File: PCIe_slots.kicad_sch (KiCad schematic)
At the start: 33 parts, among them J1 PCIe_x16_CPU

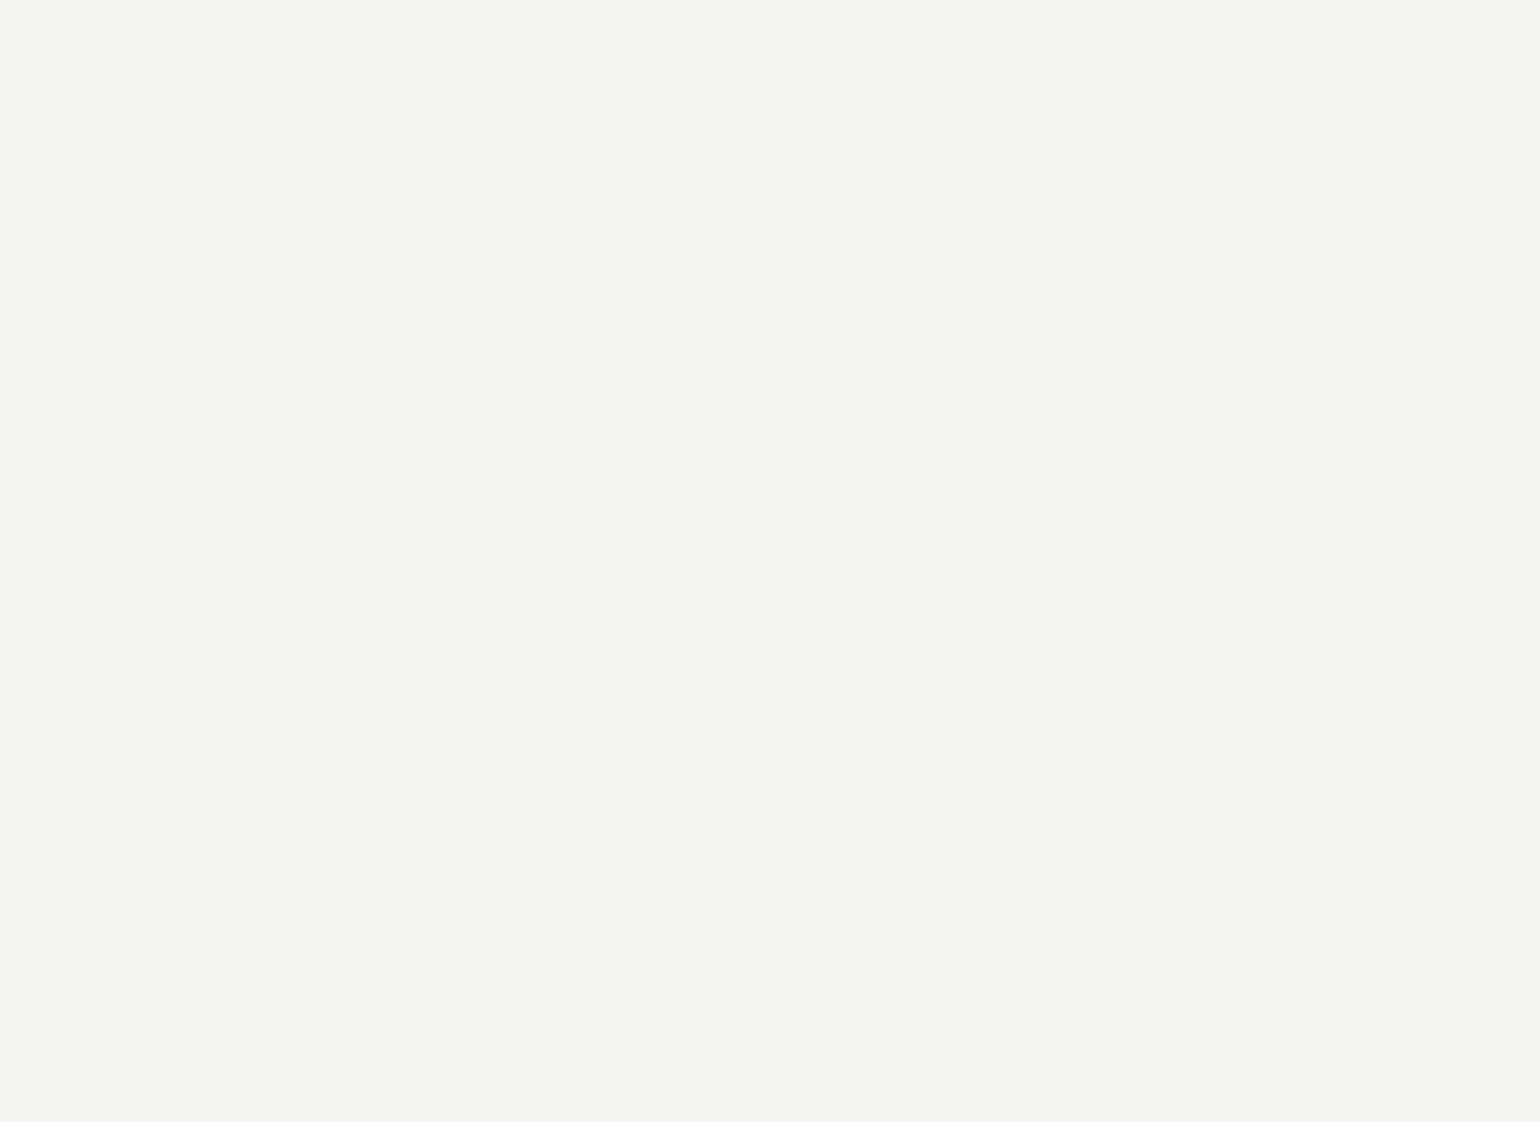
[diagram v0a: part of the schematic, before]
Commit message: idek what i changed anymore but there's a bunch of new stuff lol
iirc i did some more misc cpu pins and a bunch of pch pcie stuff
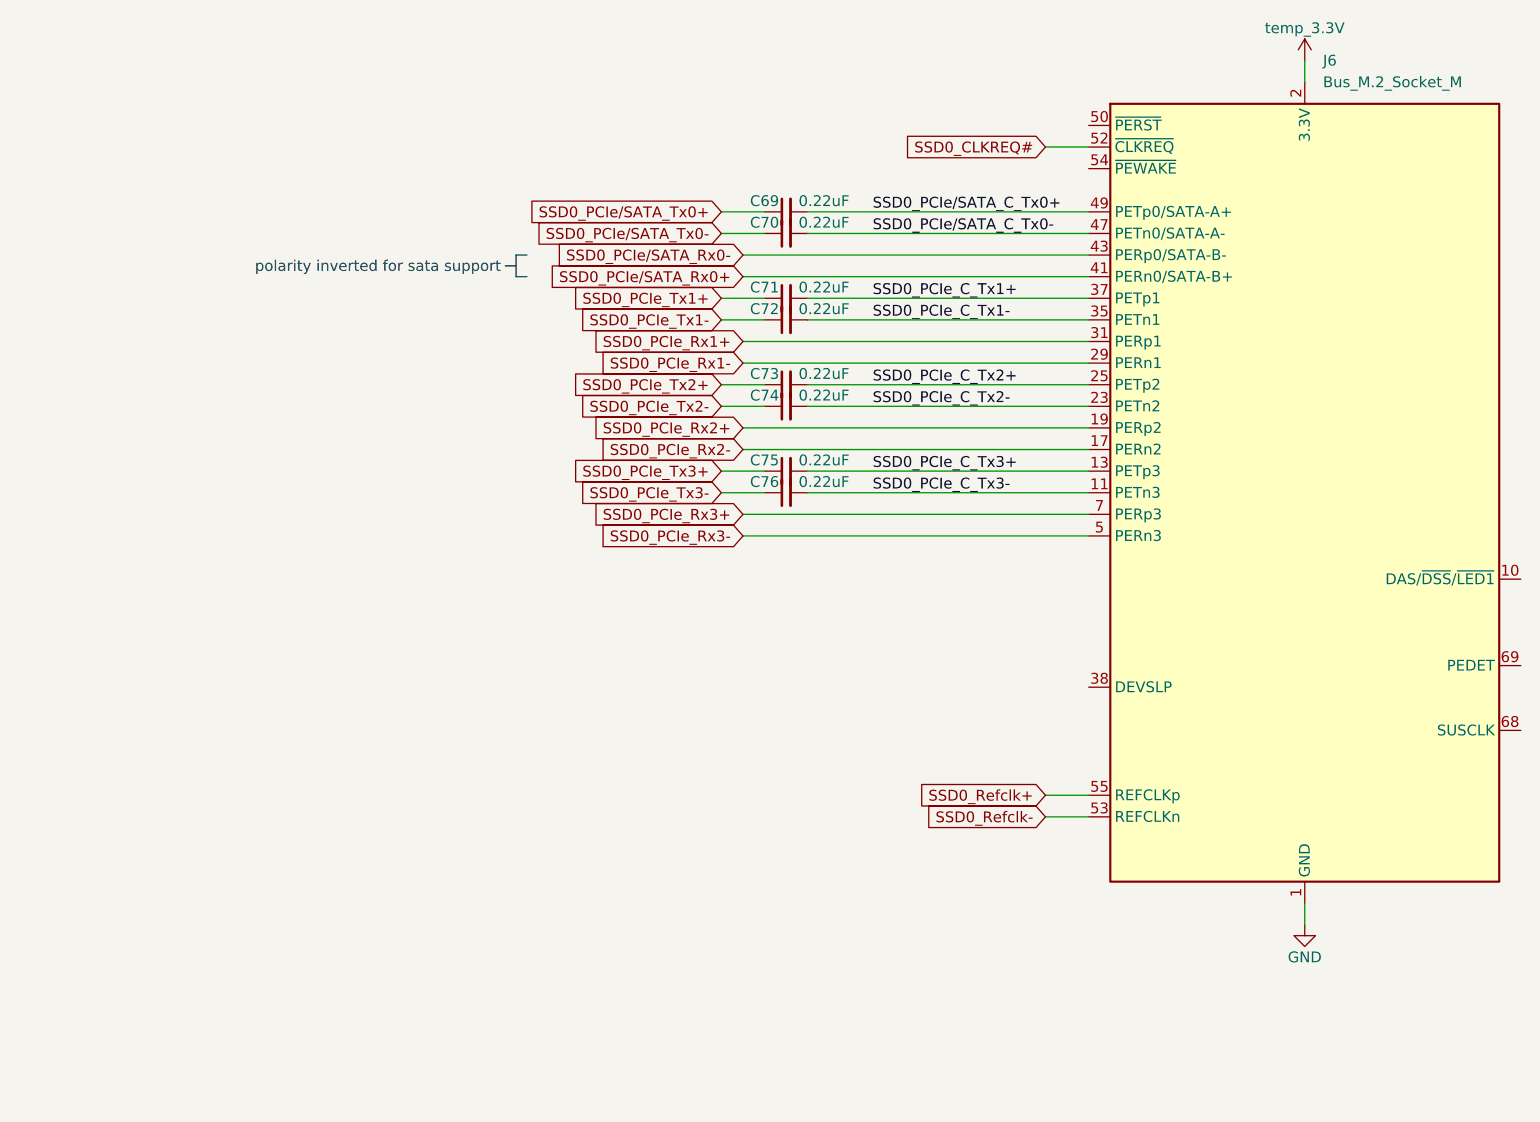
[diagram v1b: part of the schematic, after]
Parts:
- added C69, C70, C71, C72, C73, C74, C75, C76: 0.22uF, Capacitor_SMD:C_0402_1005Metric, symbol Device:C_Small
- added J6: Bus_M.2_Socket_M, A-my-stuff:m-key, symbol Connector:Bus_M.2_Socket_M
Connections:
- net GND: now also J6.1 (GND), J6.15 (GND), J6.21 (GND), J6.27 (GND), J6.3 (GND), J6.33 (GND), J6.39 (GND), J6.45 (GND), J6.51 (GND), J6.57 (GND), J6.71 (GND), J6.73 (GND), J6.75 (GND), J6.9 (GND)
- net temp_3.3V: now also J6.12 (3.3V), J6.14 (3.3V), J6.16 (3.3V), J6.18 (3.3V), J6.2 (3.3V), J6.4 (3.3V), J6.70 (3.3V), J6.72 (3.3V), J6.74 (3.3V)
- new net SSD0_CLKREQ#: J6.52 (~{CLKREQ})
- new net SSD0_PCIe/SATA_C_Tx0+: C69.2, J6.49 (PETp0/SATA-A+)
- new net SSD0_PCIe/SATA_C_Tx0-: C70.2, J6.47 (PETn0/SATA-A-)
- new net SSD0_PCIe/SATA_Rx0+: J6.41 (PERn0/SATA-B+)
- new net SSD0_PCIe/SATA_Rx0-: J6.43 (PERp0/SATA-B-)
- new net SSD0_PCIe/SATA_Tx0+: C69.1
- new net SSD0_PCIe/SATA_Tx0-: C70.1
- new net SSD0_PCIe_C_Tx1+: C71.2, J6.37 (PETp1)
- new net SSD0_PCIe_C_Tx1-: C72.2, J6.35 (PETn1)
- new net SSD0_PCIe_C_Tx2+: C73.2, J6.25 (PETp2)
- new net SSD0_PCIe_C_Tx2-: C74.2, J6.23 (PETn2)
- new net SSD0_PCIe_C_Tx3+: C75.2, J6.13 (PETp3)
- new net SSD0_PCIe_C_Tx3-: C76.2, J6.11 (PETn3)
- new net SSD0_PCIe_Rx1+: J6.31 (PERp1)
- new net SSD0_PCIe_Rx1-: J6.29 (PERn1)
- new net SSD0_PCIe_Rx2+: J6.19 (PERp2)
- new net SSD0_PCIe_Rx2-: J6.17 (PERn2)
- new net SSD0_PCIe_Rx3+: J6.7 (PERp3)
- new net SSD0_PCIe_Rx3-: J6.5 (PERn3)
- new net SSD0_PCIe_Tx1+: C71.1
- new net SSD0_PCIe_Tx1-: C72.1
- new net SSD0_PCIe_Tx2+: C73.1
- new net SSD0_PCIe_Tx2-: C74.1
- new net SSD0_PCIe_Tx3+: C75.1
- new net SSD0_PCIe_Tx3-: C76.1
- new net SSD0_Refclk+: J6.55 (REFCLKp)
- new net SSD0_Refclk-: J6.53 (REFCLKn)
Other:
- note added: "polarity inverted for sata support"
